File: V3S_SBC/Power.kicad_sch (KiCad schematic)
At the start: 15 parts, among them P1 USB_C_Plug_USB2.0, U2 EA3036CQB

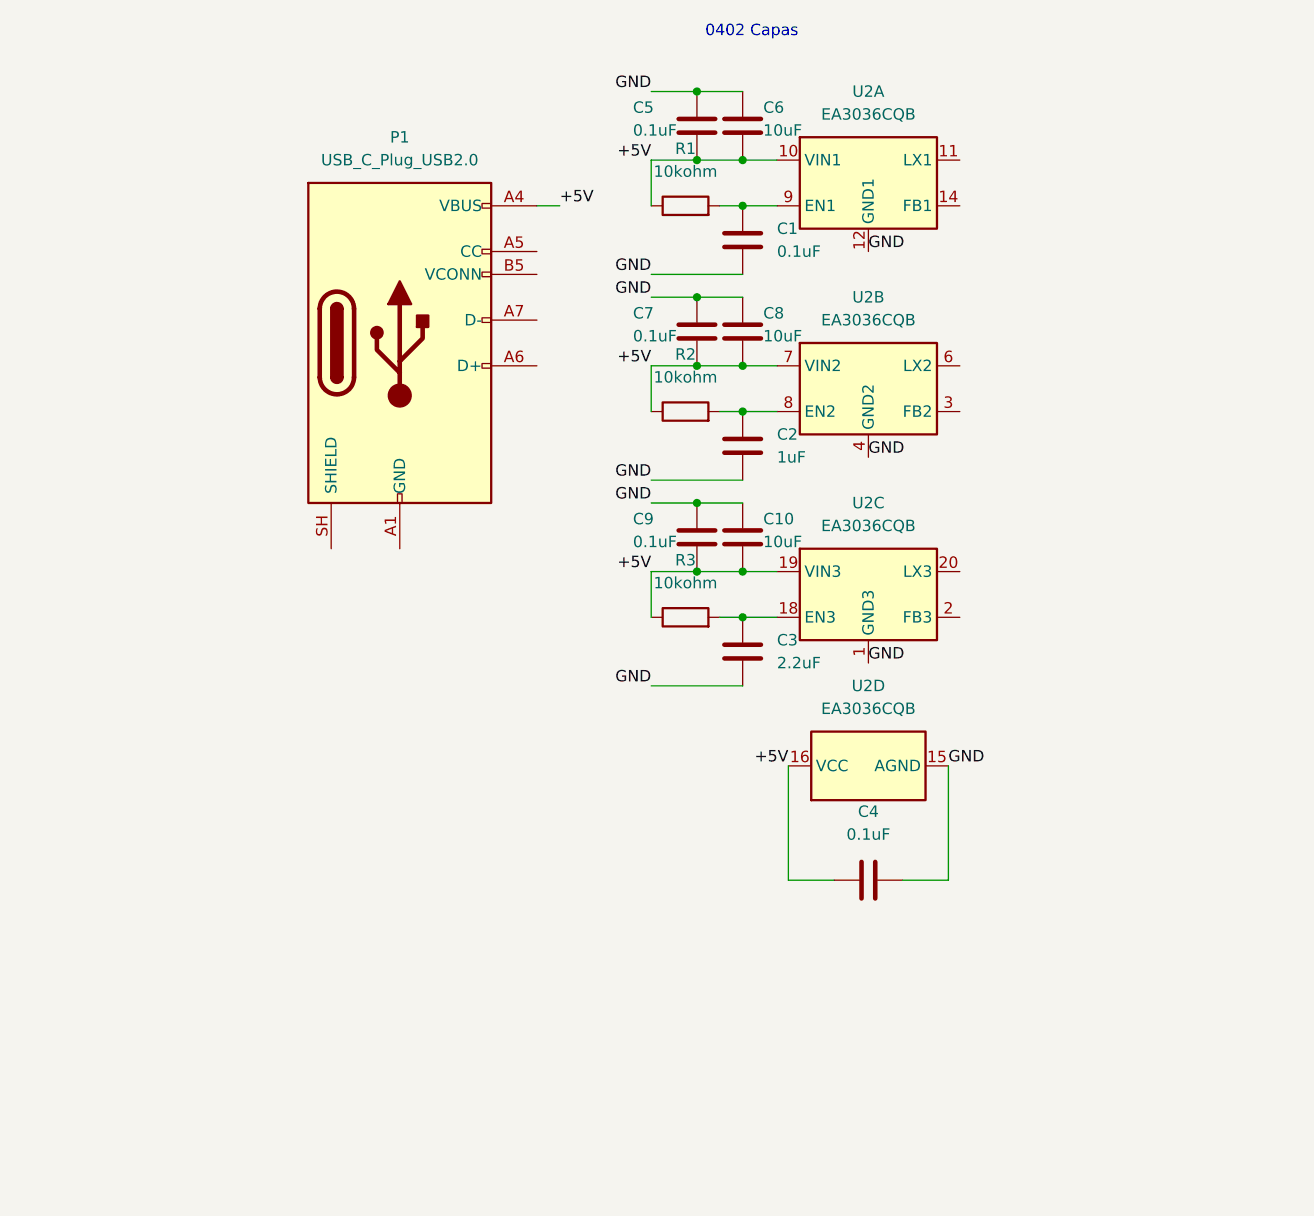
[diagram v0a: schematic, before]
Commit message: Add files via upload
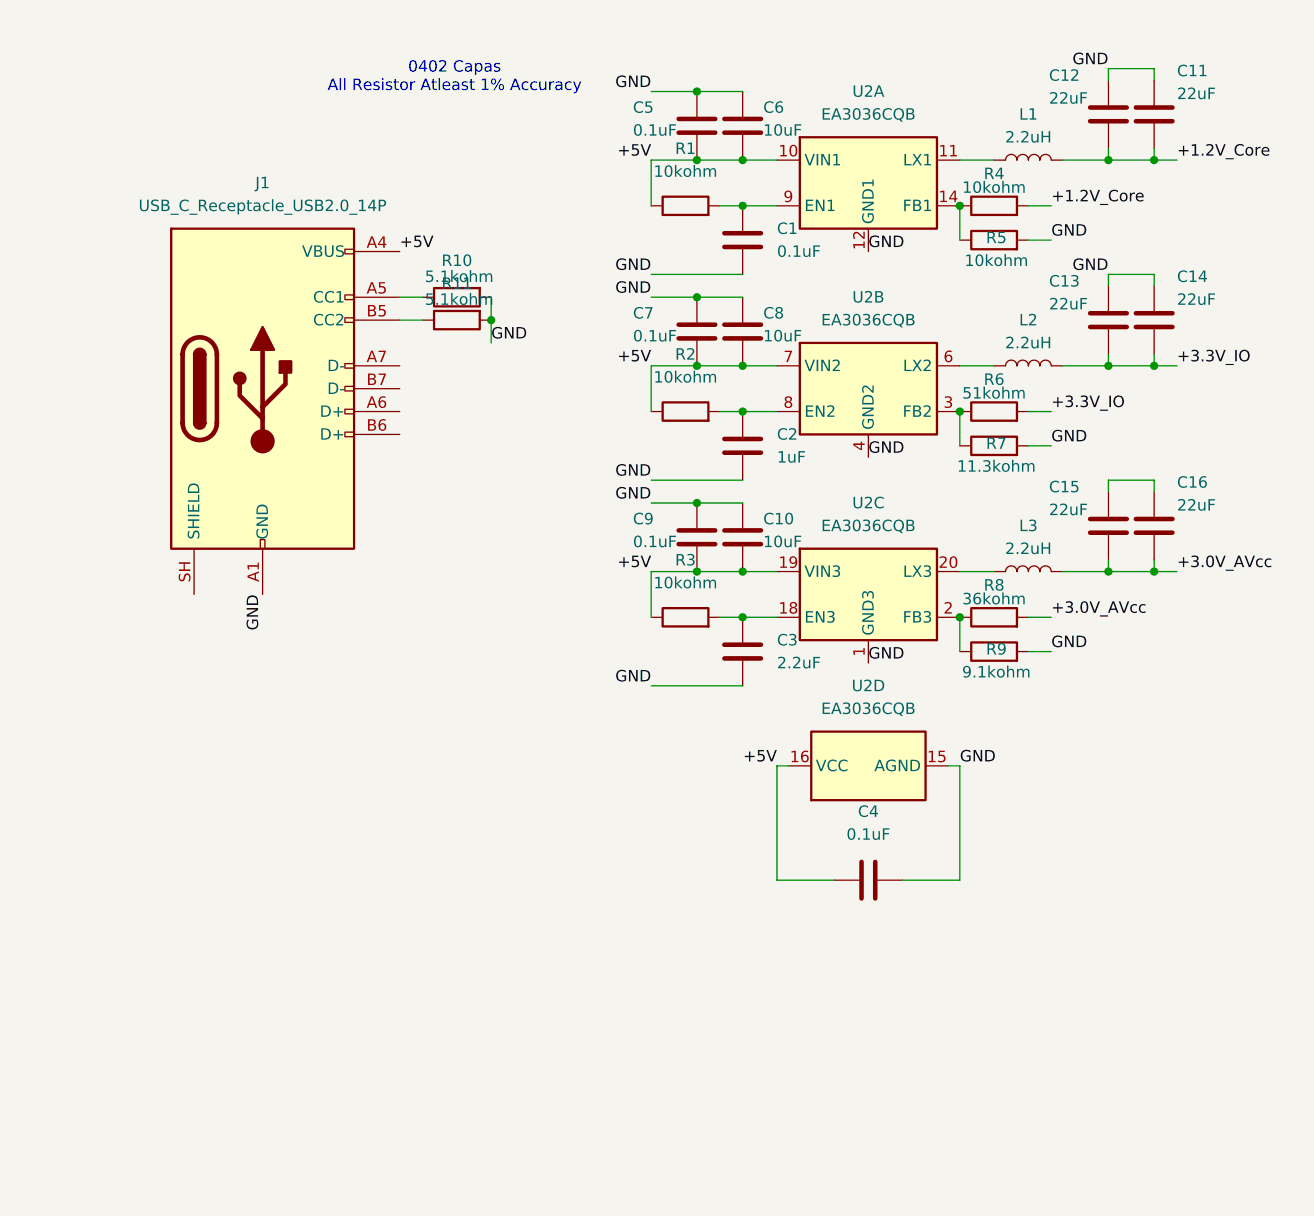
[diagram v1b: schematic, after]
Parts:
- removed P1: USB_C_Plug_USB2.0, symbol Connector:USB_C_Plug_USB2.0
- added C11, C12, C13, C14, C15, C16: 22uF, symbol Device:C
- added J1: USB_C_Receptacle_USB2.0_14P, symbol Connector:USB_C_Receptacle_USB2.0_14P
- added L1, L2, L3: 2.2uH, symbol Device:L
- added R10, R11: 5.1kohm, symbol Device:R
- added R4, R5: 10kohm, symbol Device:R
- added R6: 51kohm, symbol Device:R
- added R7: 11.3kohm, symbol Device:R
- added R8: 36kohm, symbol Device:R
- added R9: 9.1kohm, symbol Device:R
- added unit 4 of U2
- added unit 3 of U2
- added unit 2 of U2
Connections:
- net +5V: now also J1.A4 (VBUS), J1.A9 (VBUS), J1.B4 (VBUS), J1.B9 (VBUS), U2.16 (VCC), U2.19 (VIN3), U2.7 (VIN2); no longer U2.16 (VCC), U2.19 (VIN3), U2.7 (VIN2)
- net GND: now also C11.1, C12.1, C13.1, C14.1, J1.A1 (GND), J1.A12 (GND), J1.B1 (GND), J1.B12 (GND), R10.2, R11.2, R5.2, R7.2, R9.2, U2.1 (GND3), U2.15 (AGND), U2.17 (AGND), U2.21 (AGND), U2.4 (GND2), U2.5 (GND2); no longer U2.1 (GND3), U2.15 (AGND), U2.17 (AGND), U2.21 (AGND), U2.4 (GND2), U2.5 (GND2)
- net at U2.11 (LX1): now also L1.1
- net at U2.14 (FB1): now also R4.1, R5.1
- net at C3.1, R3.2: now also U2.18 (EN3); no longer U2.18 (EN3)
- net at C2.1, R2.2: now also U2.8 (EN2); no longer U2.8 (EN2)
- new net: R6.1, R7.1, U2.3 (FB2)
- new net: R8.1, R9.1, U2.2 (FB3)
- new net: L3.1, U2.20 (LX3)
- new net: L2.1, U2.6 (LX2)
- new net: J1.B5 (CC2), R11.1
- new net: C15.1, C16.1
- new net: J1.A5 (CC1), R10.1
- new net +1.2V_Core: C11.2, C12.2, L1.2, R4.2
- new net +3.0V_AVcc: C15.2, C16.2, L3.2, R8.2
- new net +3.3V_IO: C13.2, C14.2, L2.2, R6.2
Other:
- note added: "0402 Capas All Resistor Atleast 1% Accuracy"
- note removed: "0402 Capas"

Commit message: Add files via upload
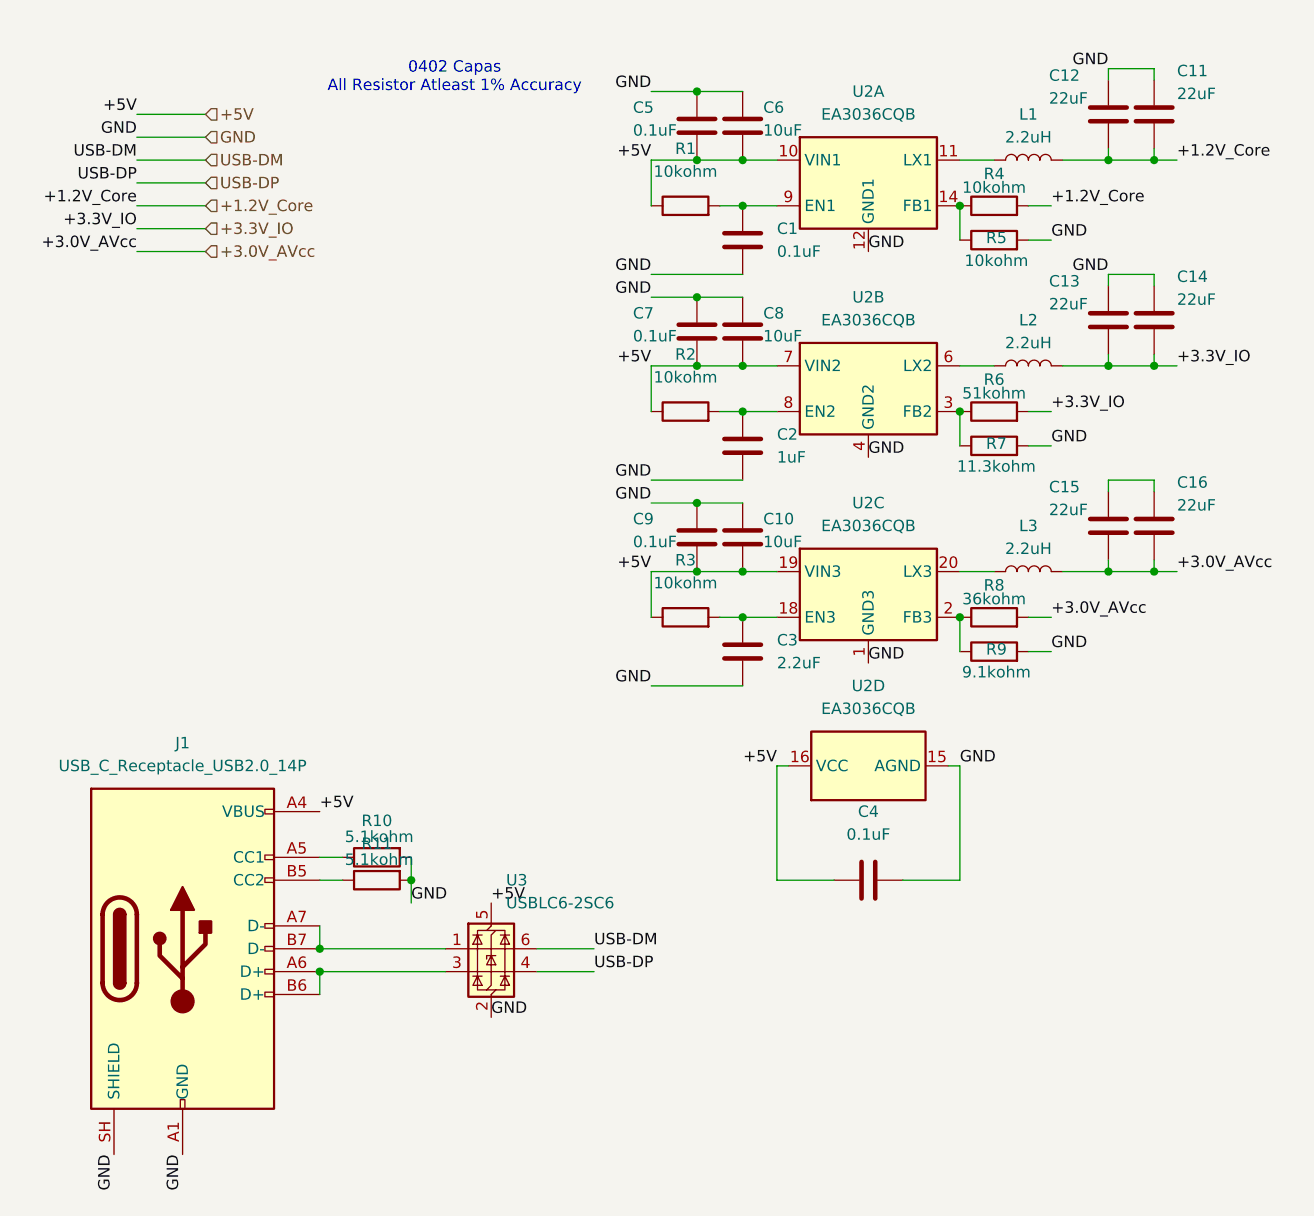
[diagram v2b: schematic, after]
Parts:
- added U3: USBLC6-2SC6, Package_TO_SOT_SMD:SOT-23-6, symbol Power_Protection:USBLC6-2SC6
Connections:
- net +5V: now also U3.5 (VBUS)
- net GND: now also J1.SH (SHIELD), U3.2 (GND)
- net at J1.A6 (D+): now also J1.B6 (D+), U3.3 (I/O2)
- net at J1.A7 (D-): now also J1.B7 (D-), U3.1 (I/O1)
- new net USB-DM: U3.6 (I/O1)
- new net USB-DP: U3.4 (I/O2)
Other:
- moved on the sheet: J1, R10, R11

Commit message: Add files via upload
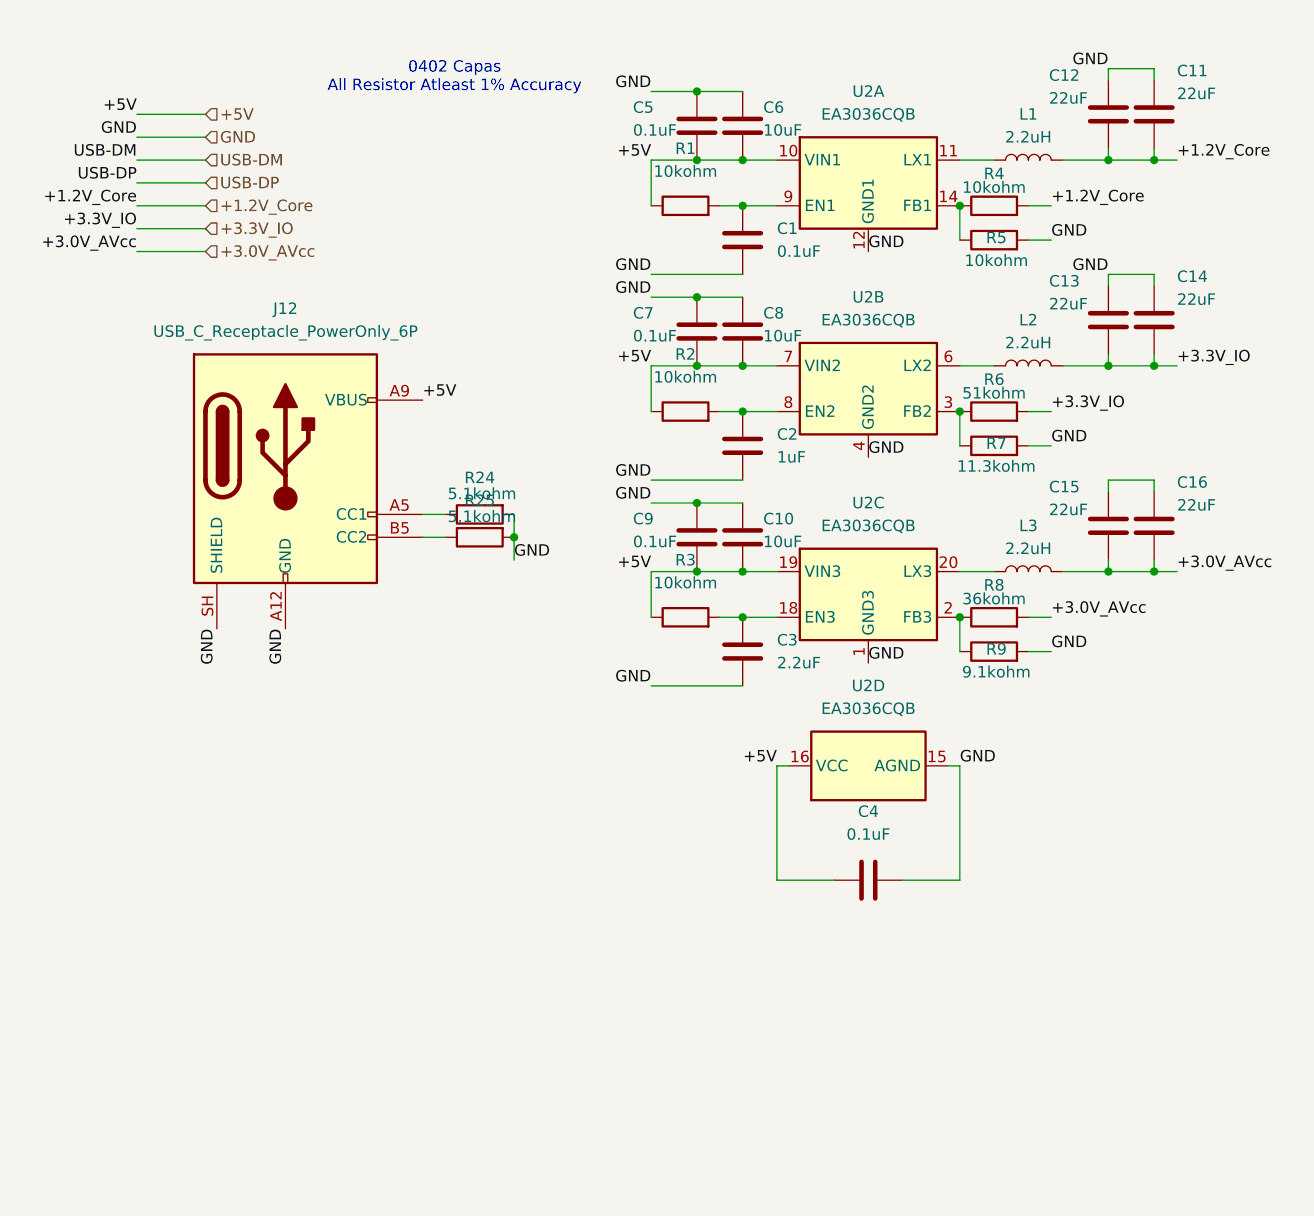
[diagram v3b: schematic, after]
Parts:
- removed J1: USB_C_Receptacle_USB2.0_14P, symbol Connector:USB_C_Receptacle_USB2.0_14P
- removed R10, R11: 5.1kohm, symbol Device:R
- removed U3: USBLC6-2SC6, Package_TO_SOT_SMD:SOT-23-6, symbol Power_Protection:USBLC6-2SC6
- added J12: USB_C_Receptacle_PowerOnly_6P, symbol Connector:USB_C_Receptacle_PowerOnly_6P
- added R24, R25: 5.1kohm, symbol Device:R
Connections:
- net +5V: now also J12.A9 (VBUS), J12.B9 (VBUS)
- net GND: now also J12.A12 (GND), J12.B12 (GND), J12.SH (SHIELD), R24.2, R25.2
- new net: J12.B5 (CC2), R25.1
- new net: J12.A5 (CC1), R24.1
